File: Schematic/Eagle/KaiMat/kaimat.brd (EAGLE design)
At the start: 60.1 x 110.5 mm, 22 parts, among them U1 THONKICONNNEW, U10 THONKICONNNEW, U11 THONKICONNNEW, U12 THONKICONNNEW, U2 THONKICONNNEW, U3 THONKICONNNEW, U4 THONKICONNNEW, U5 THONKICONNNEW, U6 THONKICONNNEW, U7 THONKICONNNEW, U8 THONKICONNNEW, U9 THONKICONNNEW

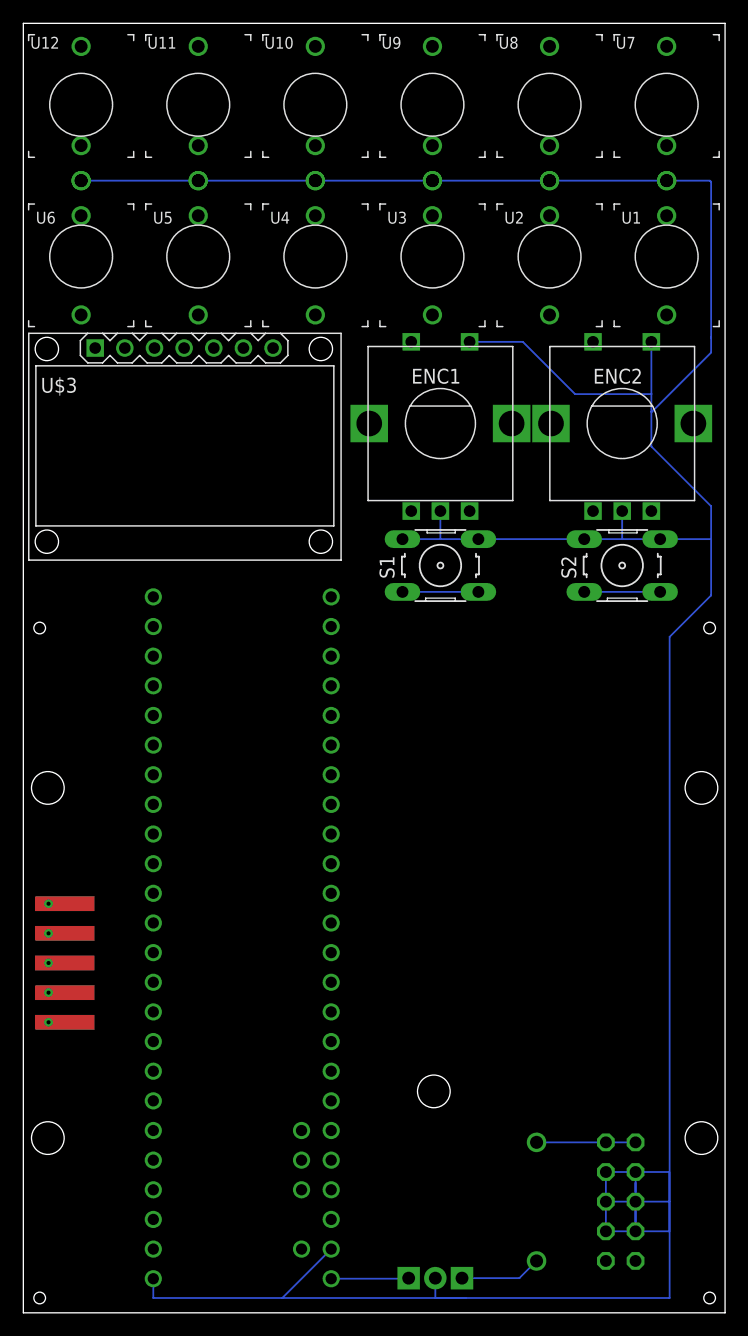
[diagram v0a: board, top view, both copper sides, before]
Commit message: pcb and eagle sch
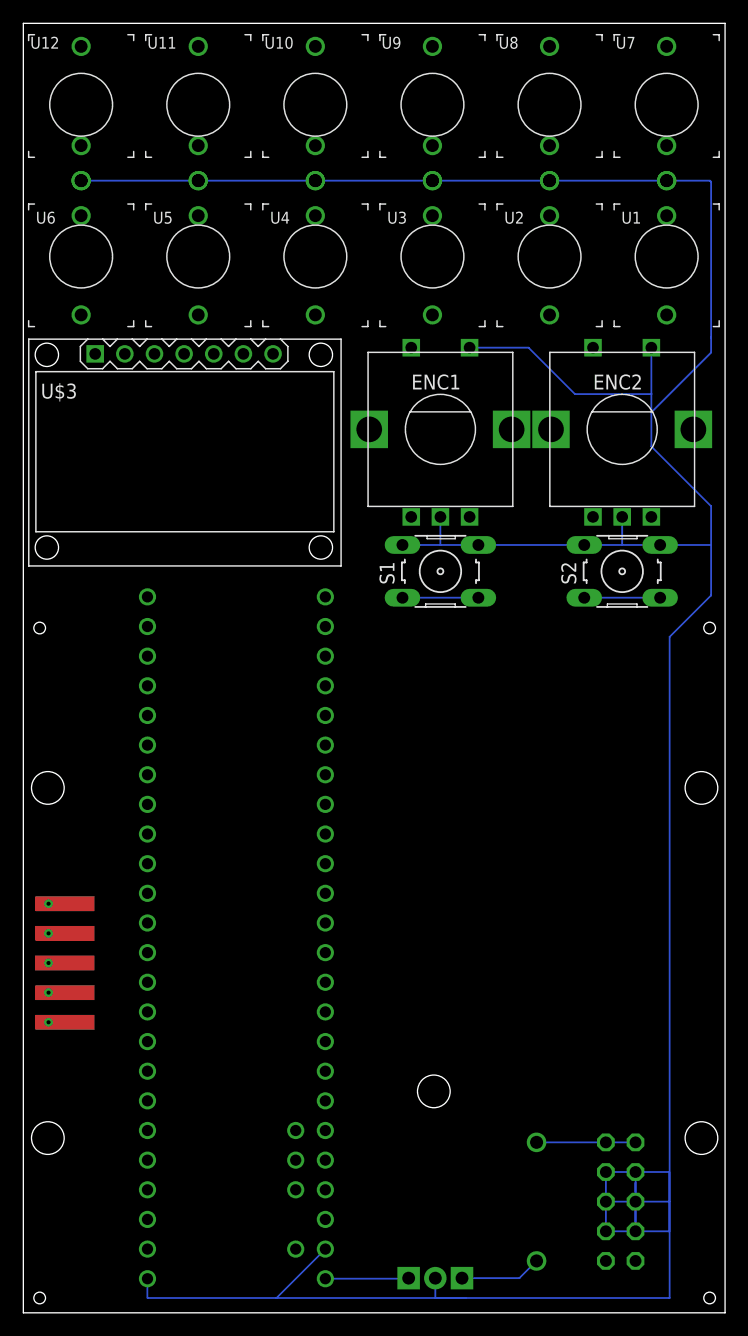
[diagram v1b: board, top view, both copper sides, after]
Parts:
- moved ENC1 0.50 mm to (35.7, 75.7)
- moved ENC2 0.50 mm to (51.3, 75.7)
- moved S1 0.50 mm to (35.7, 63.5)
- moved S2 0.50 mm to (51.3, 63.5)
- moved U$1 0.50 mm to (18.3, 30.9)
- moved U$3 0.50 mm to (13.1, 74.5)
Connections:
- removed net VCC: U$3.2
- net +5V: now also U$3.2
- net OLEDCLK: now also U$3.3
- net OLEDCS: now also U$3.7
- net OLEDDATA: now also U$3.4
- net OLEDDC: now also U$3.6
- net OLEDRST: now also U$3.5
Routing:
- net +5V: track 6.69 -> 7.19 mm
